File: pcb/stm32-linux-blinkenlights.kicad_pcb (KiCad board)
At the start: 2 copper layers, 70 x 50 mm, 42 parts, among them J1 USB_C_Receptacle, J2 Conn_01x04_Socket, SW1 SW_Push, U1 LM2575-3.3BT, U2 STM32F103C8Tx

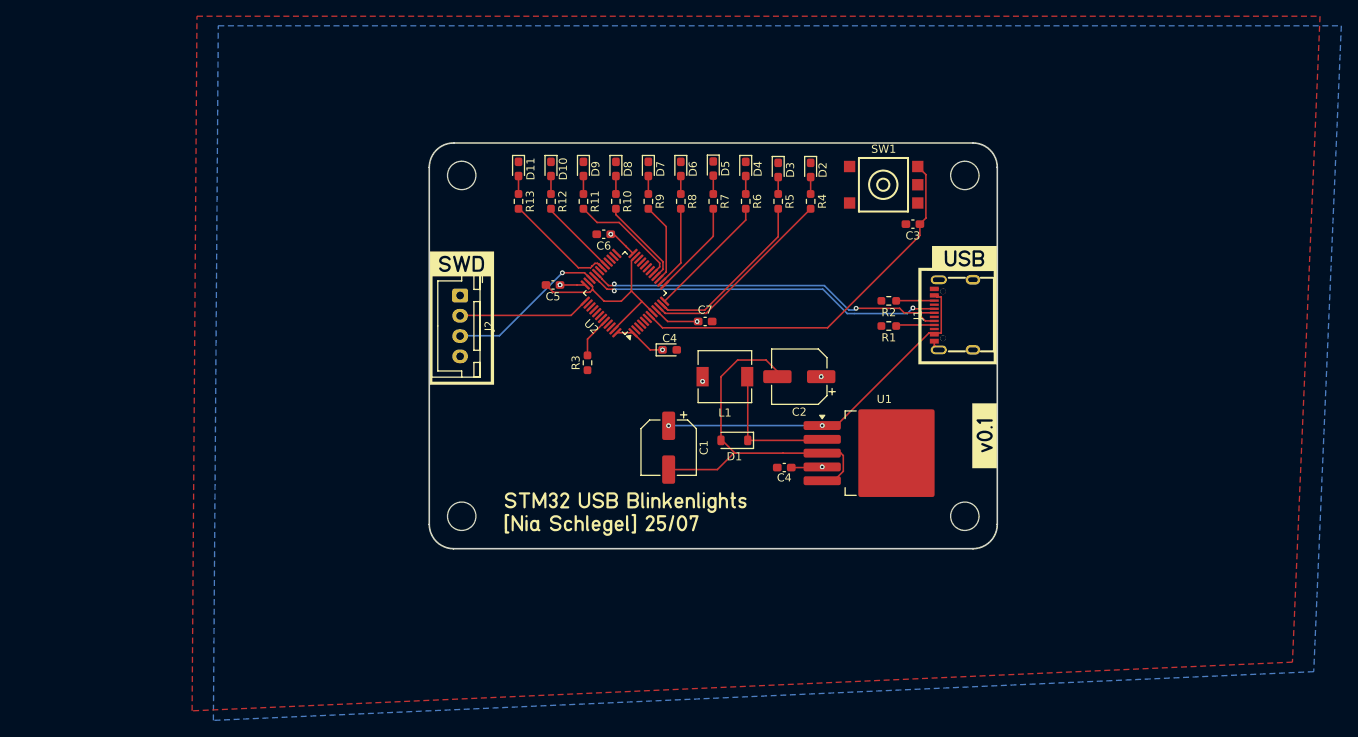
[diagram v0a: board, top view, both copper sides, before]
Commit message: v0.2?
Signed-off-by: Nia Schlegel <gott@3nt3.de>
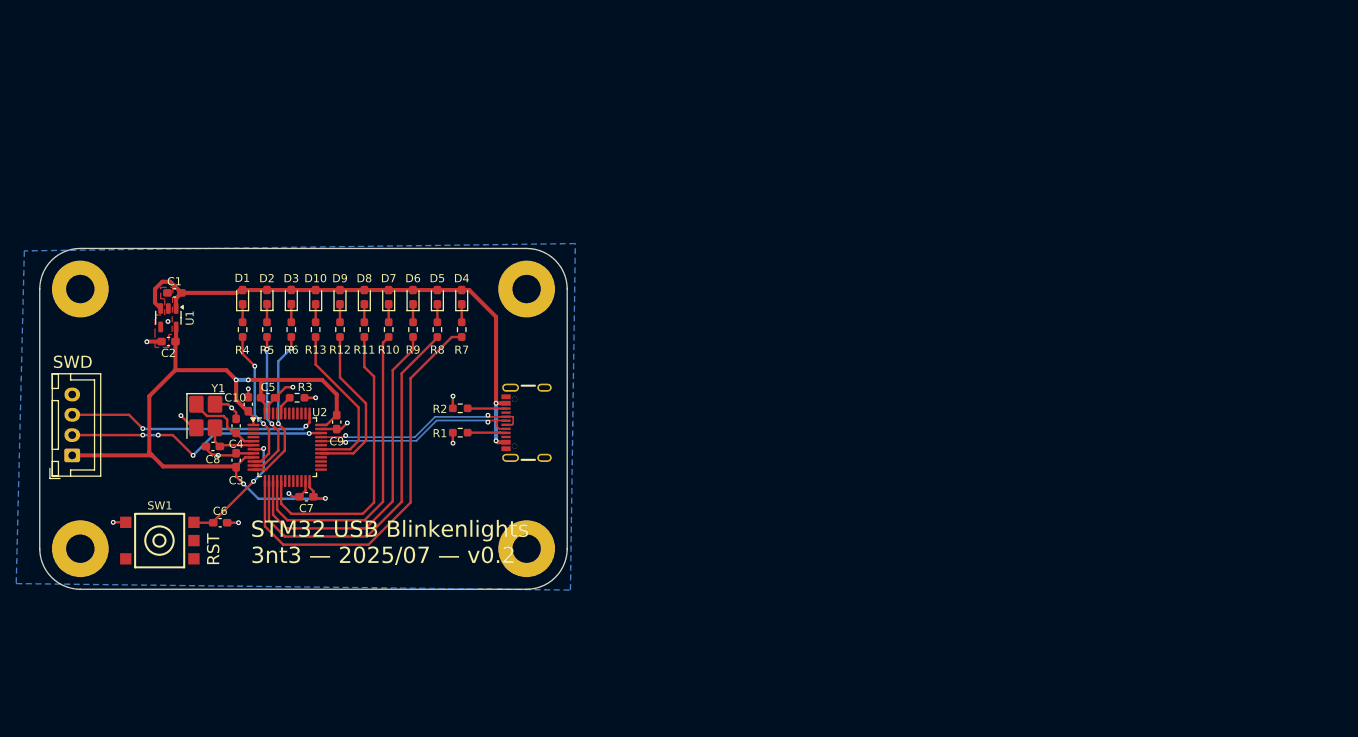
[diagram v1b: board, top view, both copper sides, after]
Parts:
- removed the C4 at (178.8, 103.0)
- removed the C4 at (164.6, 88.5)
- removed D11: LED, LED_SMD:LED_0603_1608Metric_Pad1.05x0.95mm_HandSolder
- removed L1: 330u, Inductor_SMD:L_6.3x6.3_H3
- removed REF** (x4): MountingHole_3.5mm, MountingHole:MountingHole_3.5mm
- added C10: 100n, Capacitor_SMD:C_0603_1608Metric_Pad1.08x0.95mm_HandSolder, F.Cu at (112.7, 95.2)
- added C4: 10p, Capacitor_SMD:C_0603_1608Metric_Pad1.08x0.95mm_HandSolder, F.Cu at (111.2, 97.9)
- added C8: 10p, Capacitor_SMD:C_0603_1608Metric_Pad1.08x0.95mm_HandSolder, F.Cu at (108.3, 100.4)
- added C9: 100n, Capacitor_SMD:C_0603_1608Metric_Pad1.08x0.95mm_HandSolder, F.Cu at (123.6, 97.4)
- added H1: MountingHole, MountingHole:MountingHole_3.5mm_Pad, F.Cu at (92.0, 81.0)
- added H2: MountingHole, MountingHole:MountingHole_3.5mm_Pad, F.Cu at (147.0, 113.0)
- added H3: MountingHole, MountingHole:MountingHole_3.5mm_Pad, F.Cu at (92.0, 113.0)
- added H4: MountingHole, MountingHole:MountingHole_3.5mm_Pad, F.Cu at (147.0, 81.0)
- added Y1: Crystal_GND24, Crystal:Crystal_SMD_3225-4Pin_3.2x2.5mm_HandSoldering, F.Cu at (107.5, 96.7)
- C1: value 100u -> 100n; footprint Capacitor_SMD:CP_Elec_6.3x7.7 -> Capacitor_SMD:C_0603_1608Metric_Pad1.08x0.95mm_HandSolder
- C2: value 330u -> 100n; footprint Capacitor_SMD:CP_Elec_6.3x7.7 -> Capacitor_SMD:C_0603_1608Metric_Pad1.08x0.95mm_HandSolder
- D1: value 1N5819 -> LED; footprint Diode_SMD:D_SOD-123 -> LED_SMD:LED_0603_1608Metric_Pad1.05x0.95mm_HandSolder
- J1: footprint easyeda2kicad:USB-C-SMD_TYPE-C-6PIN-2MD-073 -> easyeda2kicad:USB-C-SMD_MC-311D
- R10, R11, R12, R13, R4, R5, R6, R7, R8, R9: value 47R -> 680R
- U1: value LM2575-3.3BT -> LP5907MFX-3.3; footprint Package_TO_SOT_SMD:TO-263-5_TabPin6 -> Package_TO_SOT_SMD:SOT-23-5
- moved SW1 99.4 mm to (101.8, 112.0)
- moved U1 89.8 mm to (102.8, 84.5), turned to -90 degrees
- moved C3 88.3 mm to (111.2, 102.1), turned to 90 degrees
- moved C2 77.9 mm to (102.9, 87.5)
- moved R4 71.8 mm to (112.0, 86.0)
- moved D2 68.8 mm to (115.0, 82.0), turned to 90 degrees
- moved R5 65.0 mm to (115.0, 86.0)
- moved C1 63.8 mm to (103.6, 81.5), turned to 180 degrees
- moved D1 63.1 mm to (112.0, 82.0), turned to 90 degrees
- moved D3 62.0 mm to (118.0, 82.0), turned to 90 degrees
- moved C6 59.1 mm to (109.2, 109.8), turned to 0 degrees
- moved R6 58.2 mm to (118.0, 86.0)
- moved R2 54.4 mm to (138.8, 95.7)
- moved J1 54.4 mm to (146.8, 97.5)
- moved R1 54.4 mm to (138.8, 98.7)
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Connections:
- C1 pad 2: Net-(D1-A) -> GND
- C2 pad 2: Net-(D1-A) -> GND
- C3 pad 1: Net-(U2-NRST) -> +3.3V
- C6 pad 1: +3.3V -> Net-(U2-NRST)
- D1 pad 2: Net-(D1-A) -> VBUS
- D10 pad 1: GND -> Net-(D10-K)
- D10 pad 2: Net-(D10-A) -> VBUS
- D2 pad 1: GND -> Net-(D2-K)
- D2 pad 2: Net-(D2-A) -> VBUS
- D3 pad 1: GND -> Net-(D3-K)
- D3 pad 2: Net-(D3-A) -> VBUS
- D4 pad 1: GND -> Net-(D4-K)
- D4 pad 2: Net-(D4-A) -> VBUS
- D5 pad 1: GND -> Net-(D5-K)
- D5 pad 2: Net-(D5-A) -> VBUS
- D6 pad 1: GND -> Net-(D6-K)
- D6 pad 2: Net-(D6-A) -> VBUS
- D7 pad 1: GND -> Net-(D7-K)
- D7 pad 2: Net-(D7-A) -> VBUS
- D8 pad 1: GND -> Net-(D8-K)
- D8 pad 2: Net-(D8-A) -> VBUS
- D9 pad 1: GND -> Net-(D9-K)
- D9 pad 2: Net-(D9-A) -> VBUS
- J2 pad 2: SWCLK -> Net-(J2-Pin_2)
- J2 pad 3: SWDIO -> Net-(J2-Pin_3)
- R10 pad 1: Net-(D8-A) -> Net-(D7-K)
- R11 pad 1: Net-(D9-A) -> Net-(D8-K)
- R12 pad 1: Net-(D10-A) -> Net-(D9-K)
- R13 pad 1: Net-(D11-A) -> Net-(D10-K)
- R4 pad 1: Net-(D2-A) -> Net-(D1-K)
- R5 pad 1: Net-(D3-A) -> Net-(D2-K)
- R6 pad 1: Net-(D4-A) -> Net-(D3-K)
- R7 pad 1: Net-(D5-A) -> Net-(D4-K)
- R8 pad 1: Net-(D6-A) -> Net-(D5-K)
- R9 pad 1: Net-(D7-A) -> Net-(D6-K)
- U1 pad 2: Net-(D1-K) -> GND
- U1 pad 3: Net-(D1-A) -> VBUS
- U1 pad 4: +3.3V -> unconnected-(U1-NC-Pad4)
- U1 pad 5: Net-(D1-A) -> +3.3V
- U2 pad 34: SWDIO -> Net-(J2-Pin_2)
- U2 pad 37: SWCLK -> Net-(J2-Pin_3)
- U2 pad 5: unconnected-(U2-PD0-Pad5) -> Net-(U2-PD0)
- U2 pad 6: unconnected-(U2-PD1-Pad6) -> Net-(U2-PD1)
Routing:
- net +3.3V: track 22.9 -> 94.8 mm, vias 7 -> 4
- net Net-(D1-A): track 46.8 -> 0.00 mm
- net LED_4: track 11.9 -> 50.3 mm
- net LED_5: track 10.0 -> 45.9 mm
- net Net-(J2-Pin_2): track 0.00 -> 32.8 mm, vias 0 -> 4
- net Net-(U2-NRST): track 47.8 -> 15.4 mm, vias 0 -> 2
- net LED_6: track 9.97 -> 42.3 mm
- net Net-(J2-Pin_3): track 0.00 -> 31.4 mm, vias 0 -> 2
- net LED_7: track 11.1 -> 38.7 mm
- net VBUS: track 43.7 -> 67.2 mm
- net LED_8: track 13.8 -> 36.2 mm
- net USB_D-: track 46.3 -> 26.2 mm
- net SWDIO: track 19.7 -> 0.00 mm, vias 1 -> 0
- net USB_D+: track 44.3 -> 26.8 mm
- net SWCLK: track 16.2 -> 0.00 mm
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- added copper zone on B.Cu, net GND
- removed copper zone on B.Cu, net +3.3V
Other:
- board size 70 x 50 mm -> 65 x 42 mm
- board text added: "Eine Batstelei der Elektronikbatstelkniche Friedrichstadt 2024 e. V."
- board text added: "RST"
- board text added: "STM32 USB Blinkenlights 3nt3 — 2025/07 — v0.2"
- board text added: "SWD"
